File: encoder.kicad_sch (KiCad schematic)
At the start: 15 parts, among them SW1 RotaryEncoder_Switch_MP, U1 74LVC3G14

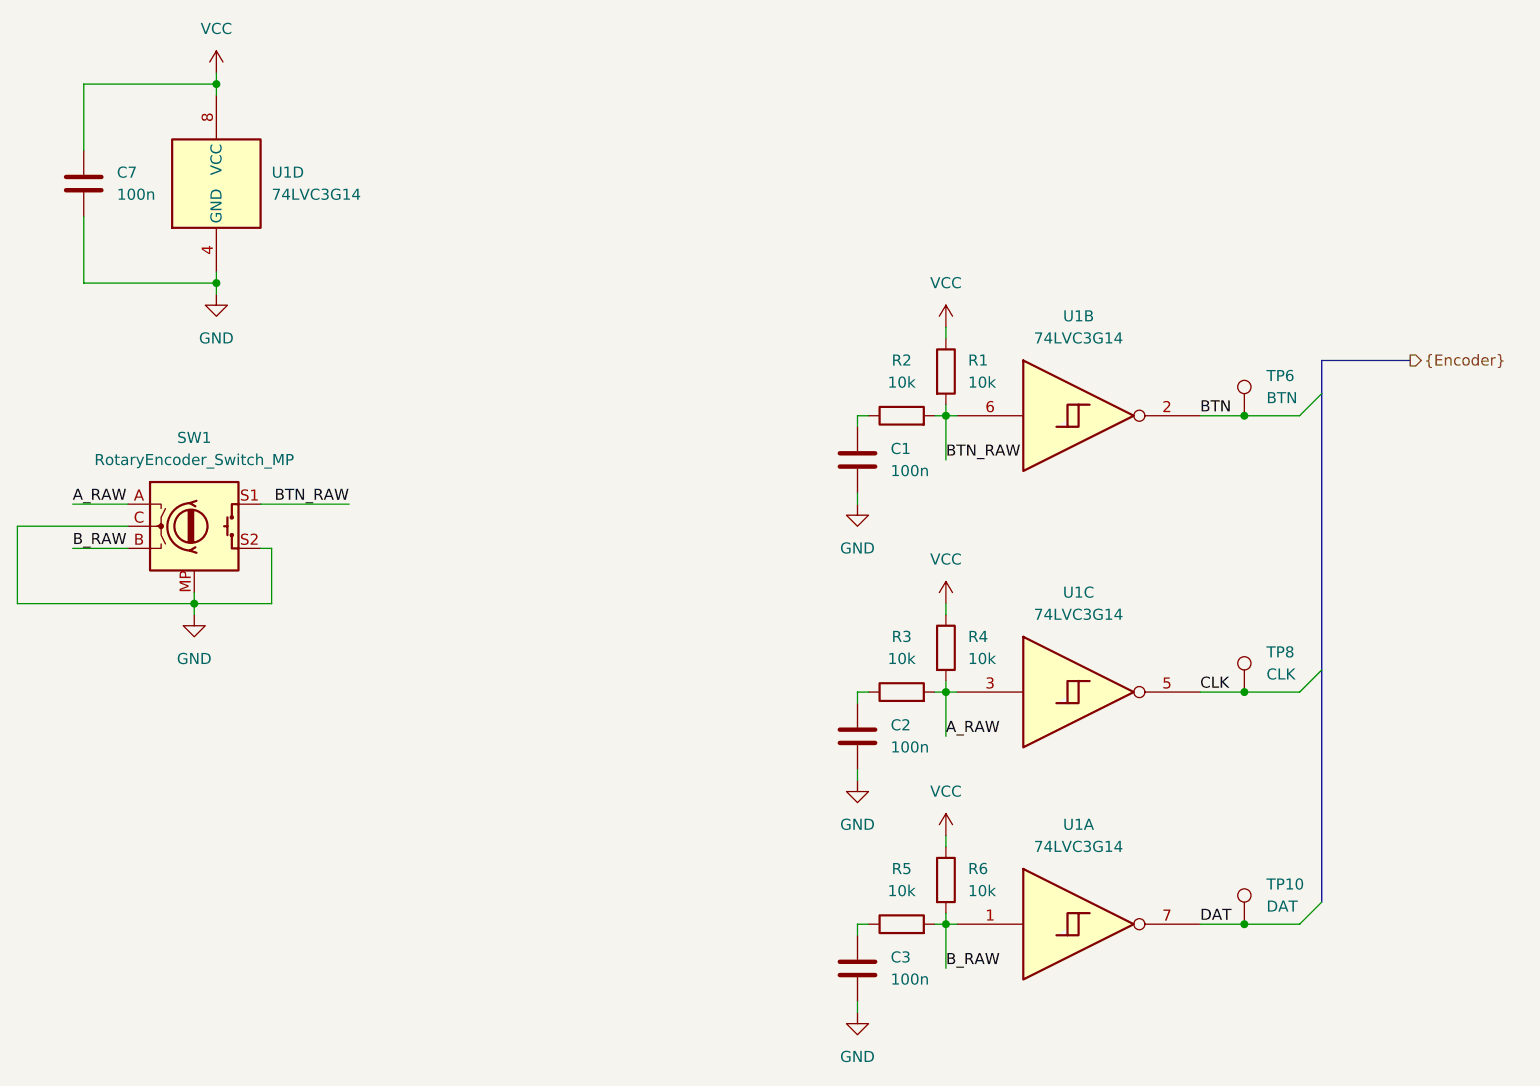
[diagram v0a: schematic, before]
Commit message: Fix encoder debounce
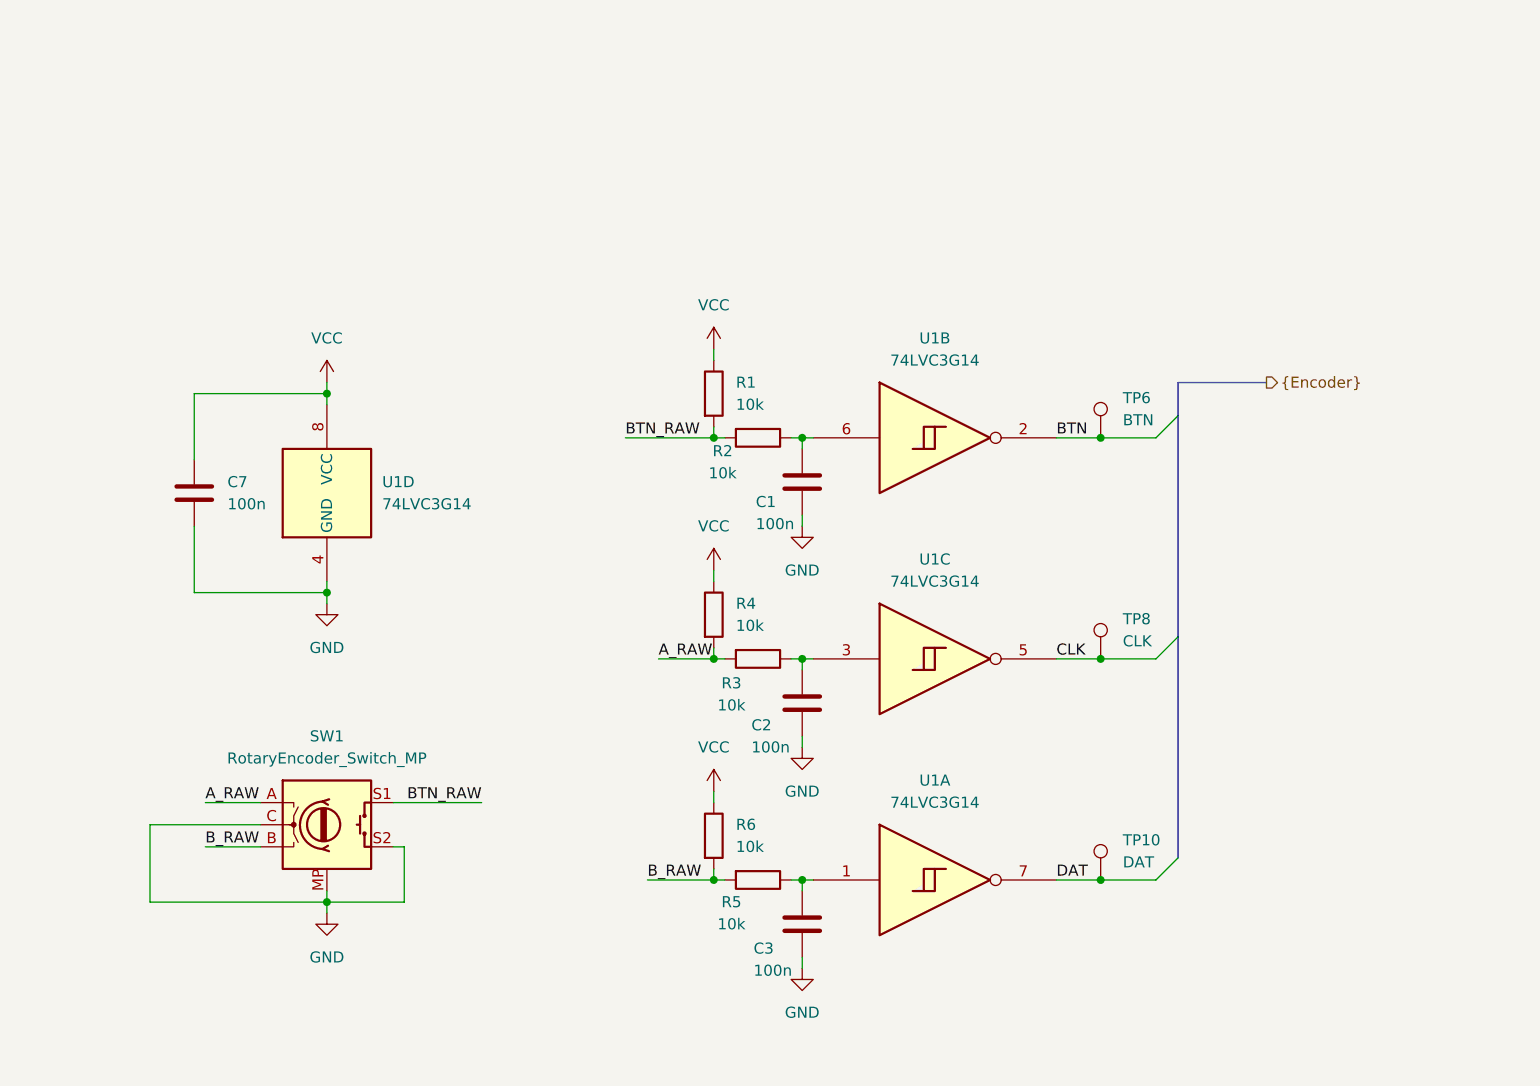
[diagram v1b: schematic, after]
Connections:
- net A_RAW: no longer U1.3
- net BTN_RAW: no longer U1.6
- net B_RAW: no longer U1.1
- net at C3.1, R5.1: now also U1.1
- net at C2.1, R3.1: now also U1.3
- net at C1.1, R2.1: now also U1.6
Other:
- moved on the sheet: C1, C2, C3, C7, R1, R2, R3, R4, R5, R6, SW1, TP10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
